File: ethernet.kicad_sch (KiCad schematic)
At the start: 32 parts, among them J1 SI-52008-F, U2 LAN8742A, Y1 ECS-3225MVLC-500-CN-TR

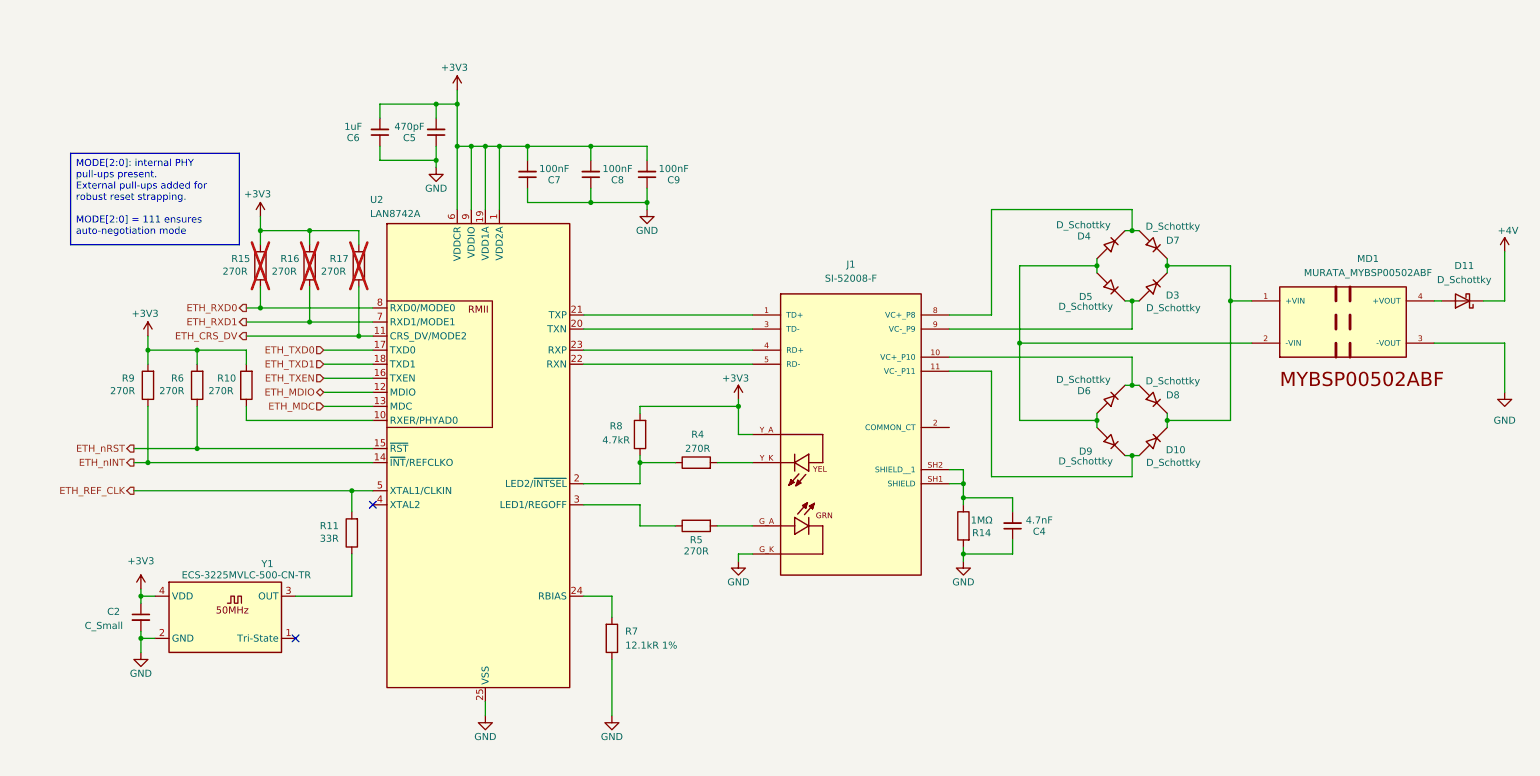
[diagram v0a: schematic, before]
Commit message: improved ETH schematics
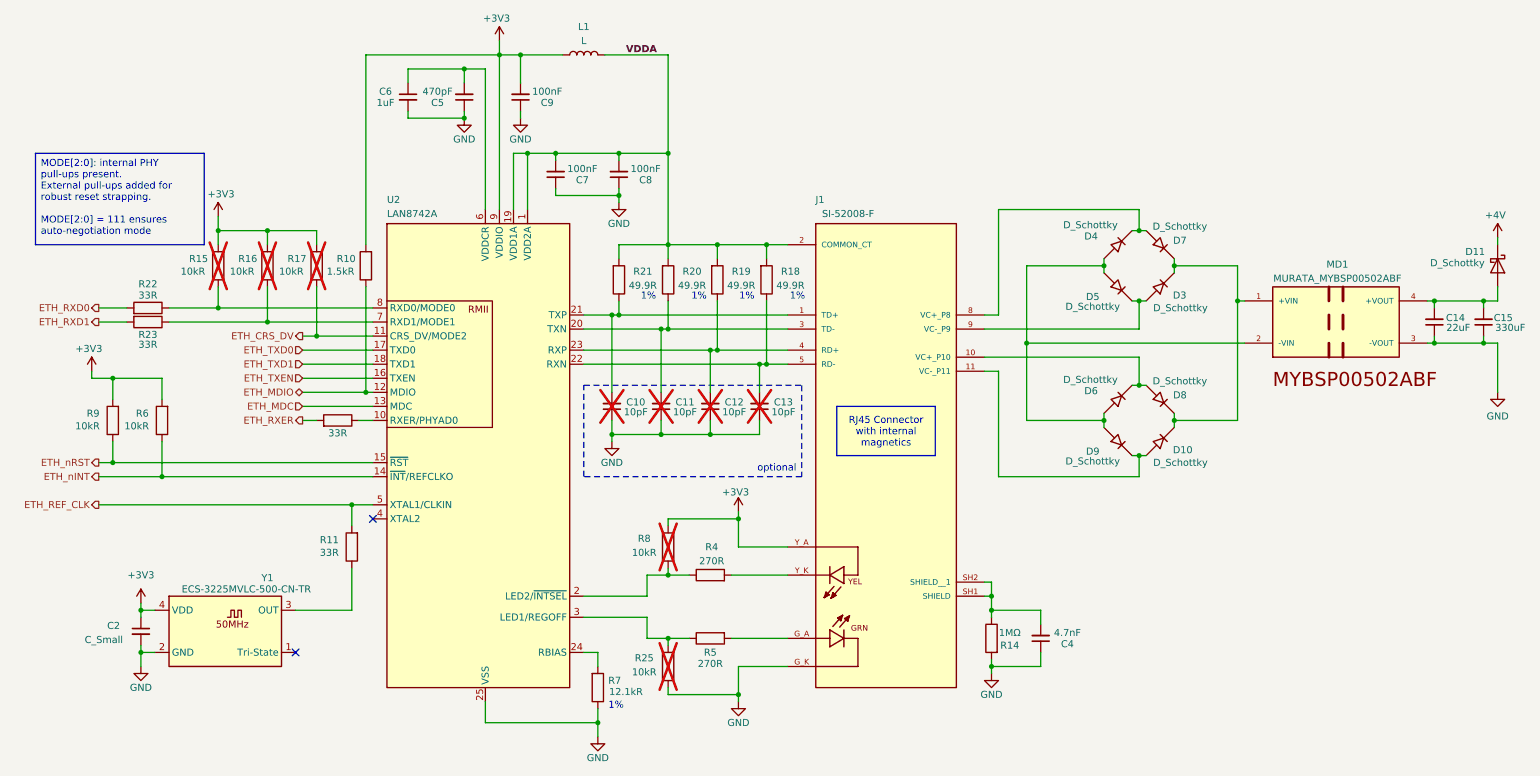
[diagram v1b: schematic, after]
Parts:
- added C10, C11, C12, C13: 10pF, Capacitor_SMD:C_0805_2012Metric_Pad1.18x1.45mm_HandSolder, symbol Device:C_Small
- added C14: 22uF, Capacitor_SMD:C_0805_2012Metric_Pad1.18x1.45mm_HandSolder, symbol Device:C_Small
- added C15: 330uF, Capacitor_SMD:C_0805_2012Metric_Pad1.18x1.45mm_HandSolder, symbol Device:C_Small
- added L1: L, symbol Device:L
- added R18, R19, R20, R21: 49.9R, Resistor_SMD:R_0805_2012Metric_Pad1.20x1.40mm_HandSolder, symbol Device:R
- added R22, R23, R24: 33R, Resistor_SMD:R_0805_2012Metric_Pad1.20x1.40mm_HandSolder, symbol Device:R
- added R25: 10kR, Resistor_SMD:R_0805_2012Metric_Pad1.20x1.40mm_HandSolder, symbol Device:R
- R10: value 270R -> 1.5kR
- R15, R16, R17, R6, R9: value 270R -> 10kR
- R7: value 12.1kR 1% -> 12.1kR
- R8: value 4.7kR -> 10kR; now not fitted
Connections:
- net +3V3: now also L1.1; no longer C5.2, C6.2, C7.2, C8.2, U2.1 (VDD2A), U2.19 (VDD1A), U2.6 (VDDCR)
- net ETH_MDIO: now also R10.1
- net ETH_RXD0: now also R22.2; no longer R15.1, U2.8 (RXD0/MODE0)
- net ETH_RXD1: now also R23.2; no longer R16.1, U2.7 (RXD1/MODE1)
- net ETH_nINT: now also R6.1; no longer R9.1
- net ETH_nRST: now also R9.1; no longer R6.1
- net GND: now also C6.2, C10.1, C11.1, C12.1, C13.1, C14.1, C15.1, R25.1; no longer C6.1
- net at U2.10 (RXER/PHYAD0): now also R24.1; no longer R10.1
- net at J1.3 (TD-), U2.20 (TXN): now also C11.2, R20.1
- net at J1.1 (TD+), U2.21 (TXP): now also C10.2, R21.1
- net at J1.5 (RD-), U2.22 (RXN): now also C13.2, R18.1
- net at J1.4 (RD+), U2.23 (RXP): now also C12.2, R19.1
- net at R5.1, U2.3 (LED1/REGOFF): now also R25.2
- net VDDA: now reaches J1.2 (COMMON_CT)
- net VDDA: now also C7.2, C8.2, U2.1 (VDD2A), U2.19 (VDD1A), L1.2, R18.2, R19.2, R20.2, R21.2
- net at D11.2 (A), MD1.4 (+VOUT): now also C14.2, C15.2
- new net: C5.2, C6.1, U2.6 (VDDCR)
- new net: R16.1, R23.1, U2.7 (RXD1/MODE1)
- new net: R15.1, R22.1, U2.8 (RXD0/MODE0)
- new net ETH_RXER: R24.2
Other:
- note added: "1%"
- moved on the sheet: C2, C4, C5, C6, C7, C8, C9, D10, D11, D3, D4, D5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
